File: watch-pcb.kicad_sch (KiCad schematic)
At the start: 0 parts

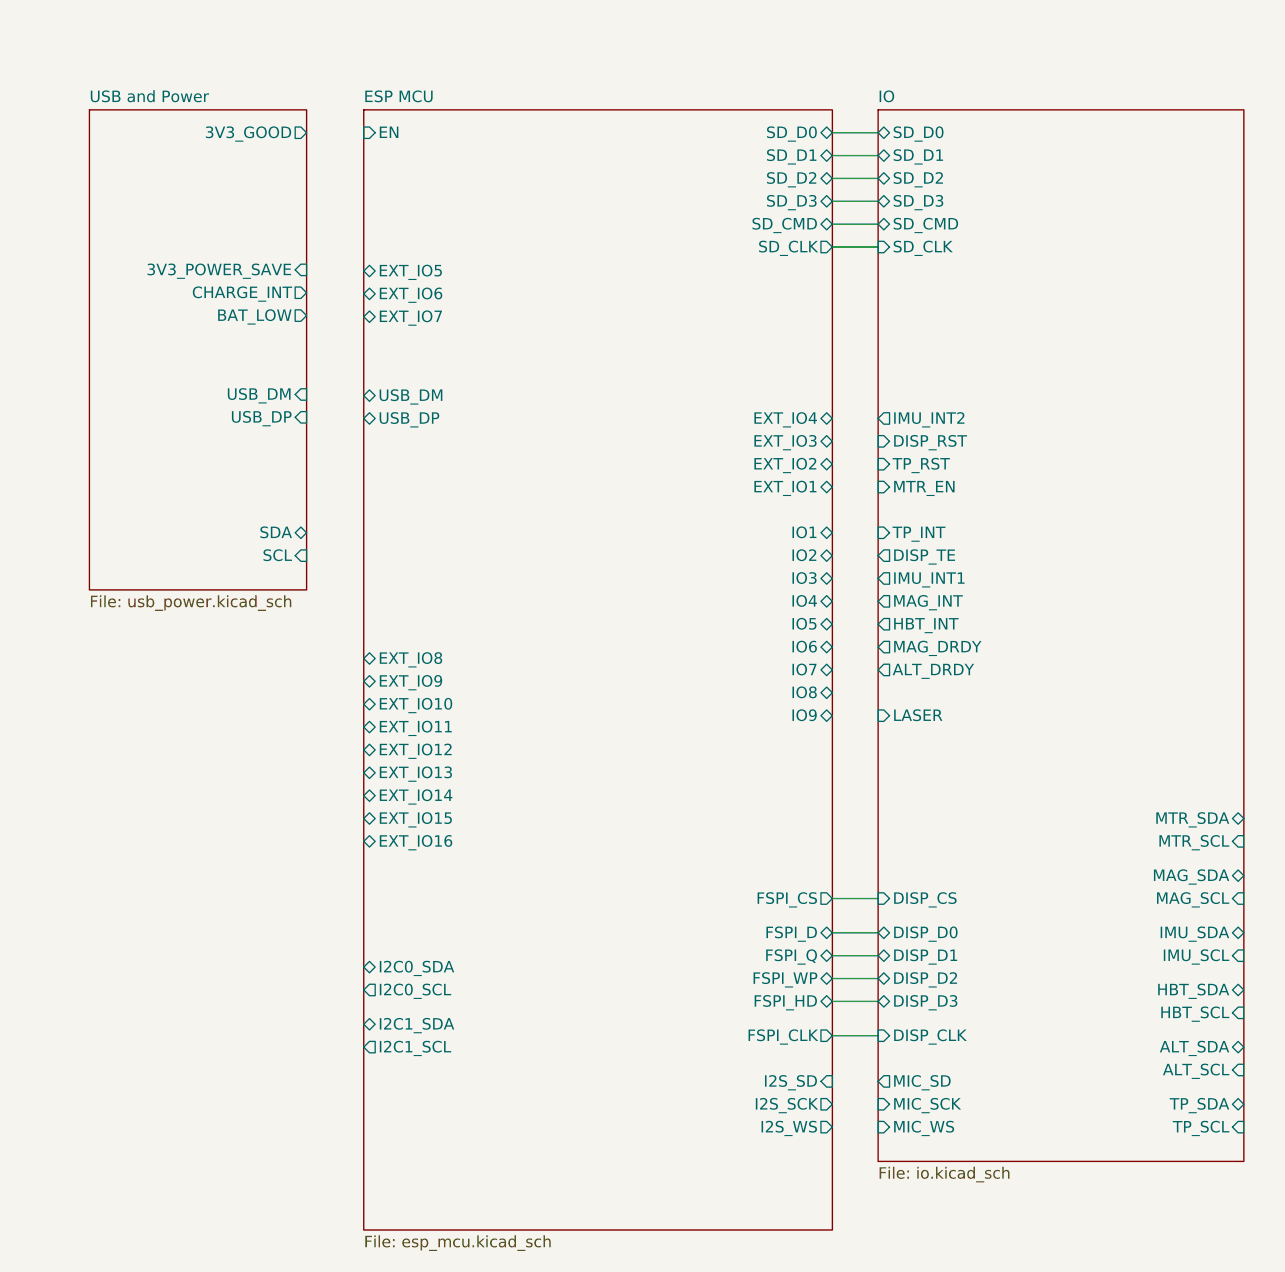
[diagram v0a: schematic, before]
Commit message: layout done probably
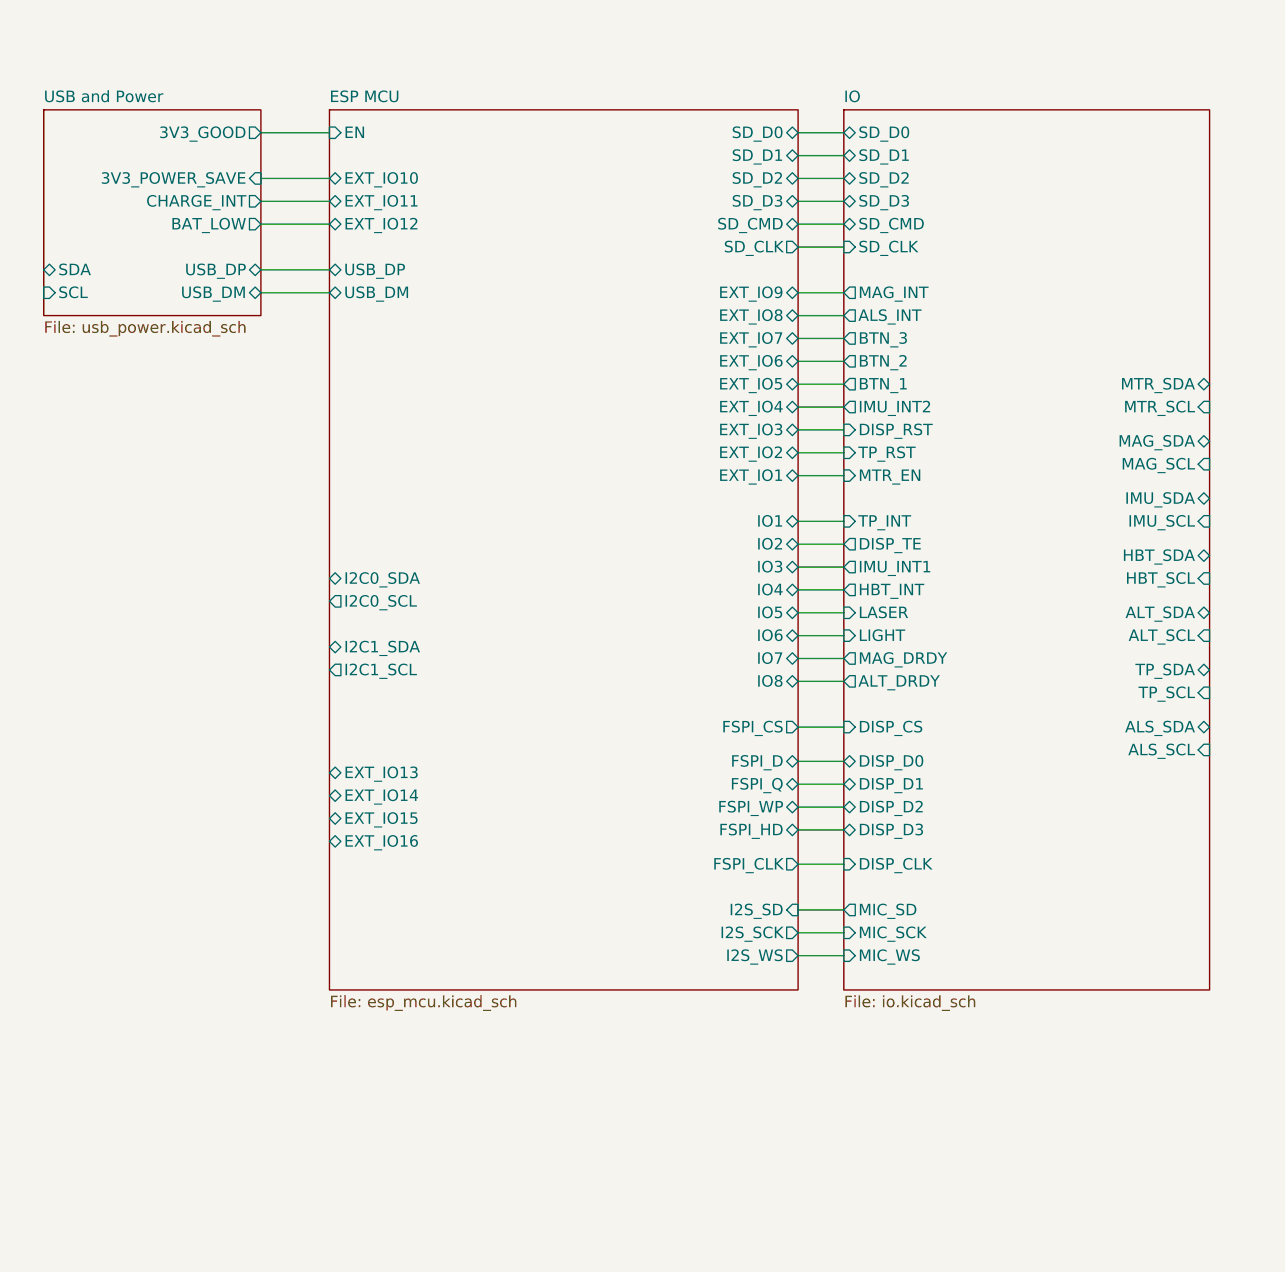
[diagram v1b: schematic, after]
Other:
- sheet ESP MCU ports: added none; removed IO9
- sheet IO ports: added ALS_INT, ALS_SCL, ALS_SDA, BTN_1, BTN_2, BTN_3, LIGHT; removed none

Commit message: finally routed the memory :D
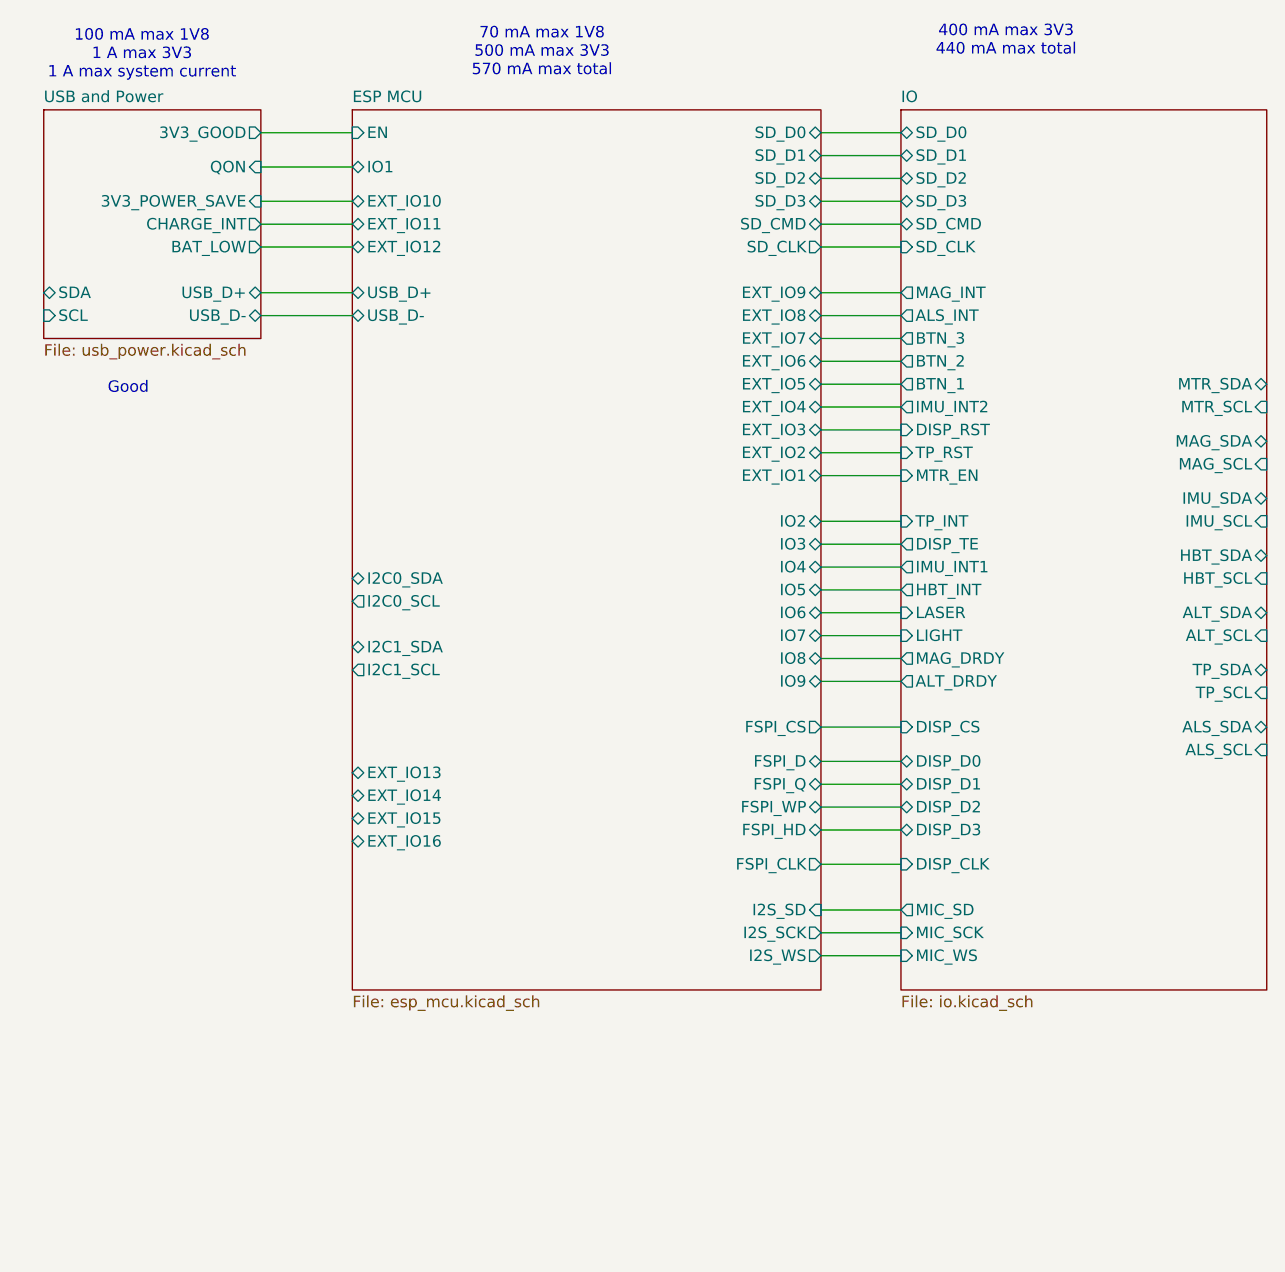
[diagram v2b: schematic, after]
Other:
- sheet ESP MCU ports: added IO9, USB_D+, USB_D-; removed USB_DM, USB_DP
- sheet USB and Power ports: added QON, USB_D+, USB_D-; removed USB_DM, USB_DP
- note added: "100 mA max 1V8 1 A max 3V3 1 A max system current"
- note added: "400 mA max 3V3 440 mA max total"
- note added: "70 mA max 1V8 500 mA max 3V3 570 mA max total"
- note added: "Good"
